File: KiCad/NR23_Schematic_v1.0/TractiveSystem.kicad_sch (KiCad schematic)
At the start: 32 parts, among them M1 Zero_7R_Motor

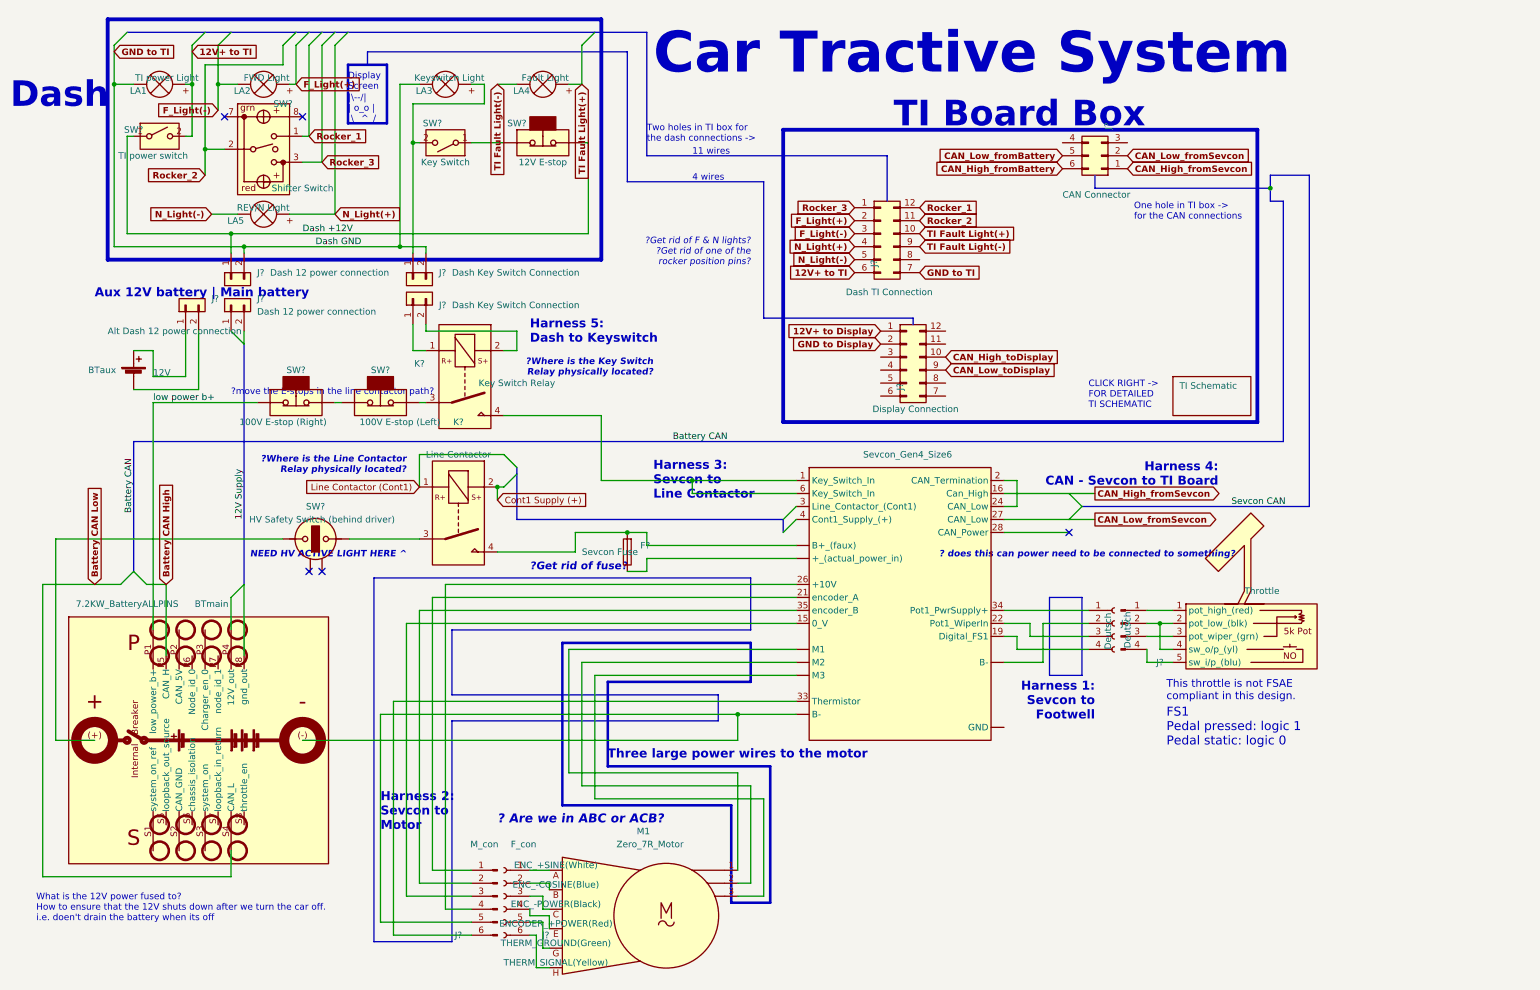
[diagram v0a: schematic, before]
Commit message: start of class 18APR23
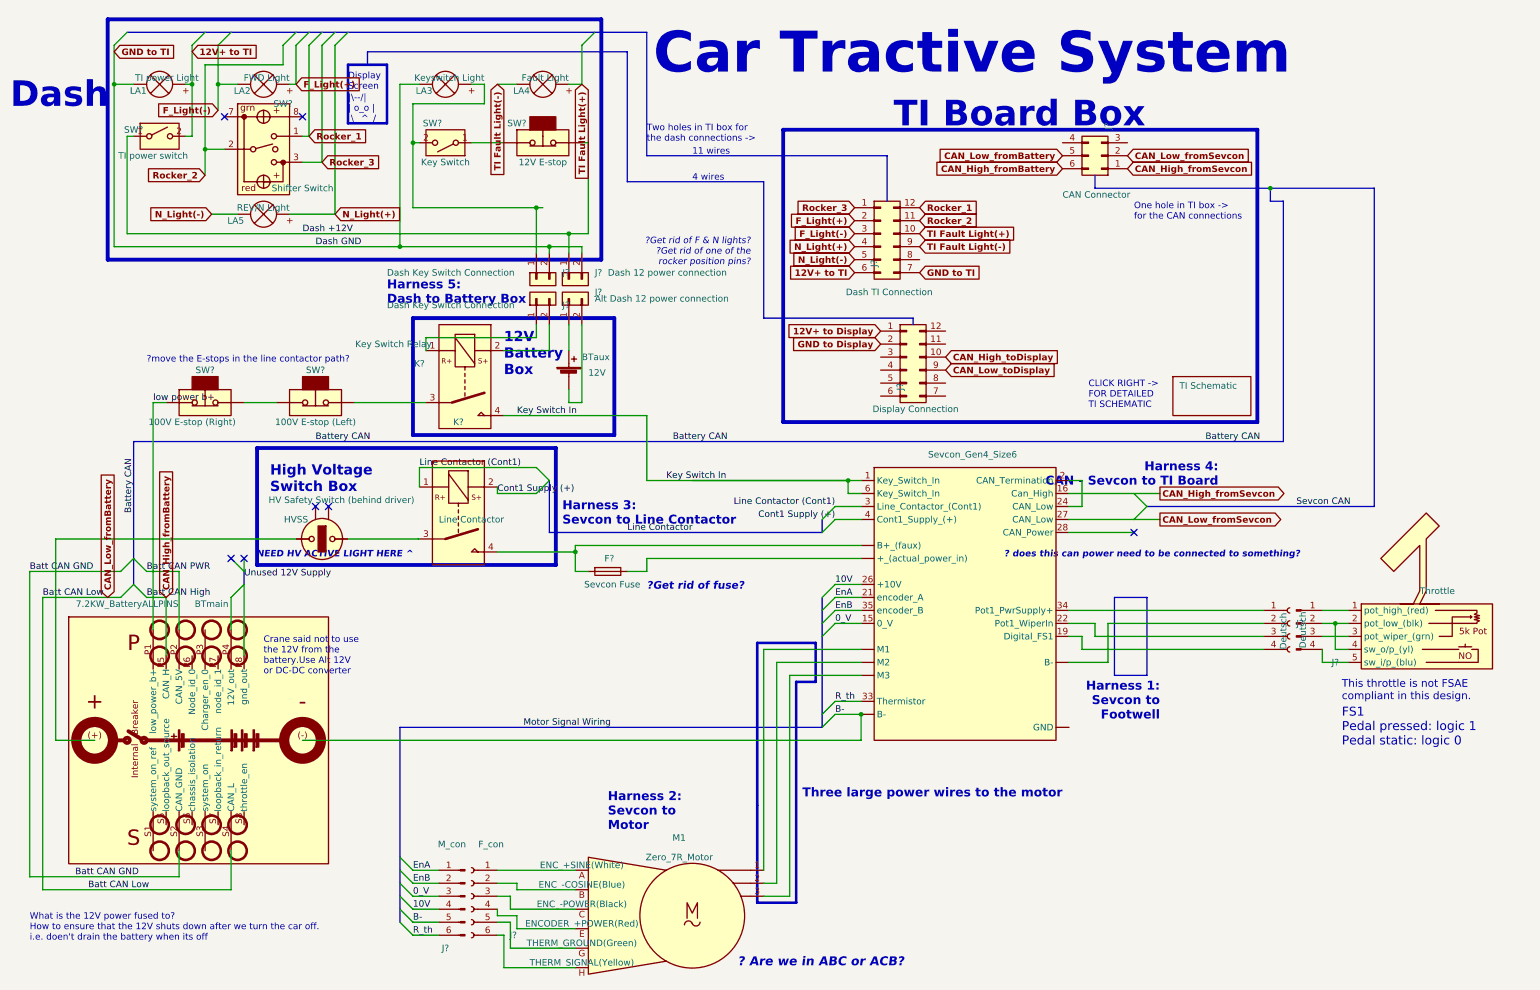
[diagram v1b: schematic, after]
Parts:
- removed J?: Dash 12 power connection, symbol Connector_Generic:Conn_01x02
- gave numbers to parts that had none: 1
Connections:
- net Battery CAN High is gone; now on net CAN_High_fromBattery: BTmain.P5 (CAN_H)
- net Battery CAN Low is gone; now on net CAN_Low_fromBattery: BTmain.S4 (CAN_L)
- net Cont1 Supply (+): now also U?.4 (Cont1_Supply_(+))
- net Line Contactor (Cont1): now also U?.3 (Line_Contactor_(Cont1))
- net EnA: now reaches J?.1 (Pin_1), U?.21 (encoder_A)
- net EnB: now reaches J?.2 (Pin_2), U?.35 (encoder_B)
- net 0_V: now reaches J?.3 (Pin_3), U?.15 (0_V)
- net 10V: now reaches J?.4 (Pin_4), U?.26 (+10V)
- net B-: now reaches BTmain.(-), J?.5 (Pin_5), U?. (M3)
- net R_th: now reaches J?.6 (Pin_6), U?.33 (Thermistor)
- net Key Switch In: now reaches K?.4, U?.1 (Key_Switch_In), U?.6 (Key_Switch_In)
- net at BTmain.(+): now also HVSS.2 (B); no longer HVSS.1 (A)
- net Batt CAN PWR: now reaches BTmain.P2 (CAN_5V)
- net Batt CAN GND: now reaches BTmain.S2 (CAN_GND)
- net at K?.3: now also HVSS.1 (A); no longer HVSS.2 (B)
- no-connect marks 5 -> 7
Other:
- note added: "12V Battery Box"
- note added: "Crane said not to use the 12V from the battery.Use Alt 12V or DC-DC converter"
- note added: "Harness 5: Dash to Battery Box"
- note added: "High Voltage Switch Box"
- note removed: "?Where is the Key Switch Relay physically located?"
- note removed: "?Where is the Line Contactor Relay physically located?"
- note removed: "Aux 12V battery | Main battery"
- note removed: "Harness 5: Dash to Keyswitch"
- moved on the sheet: BTaux, F?, HVSS, J?, M1, SW?
